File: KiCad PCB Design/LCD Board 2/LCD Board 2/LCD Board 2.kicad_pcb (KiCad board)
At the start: 2 copper layers, 27.9 x 27.9 mm, 8 parts, among them J1 Conn_01x03_Male, J2 Conn_01x03_Male, J3 Conn_01x02_Male, U1 ATtiny412-SS

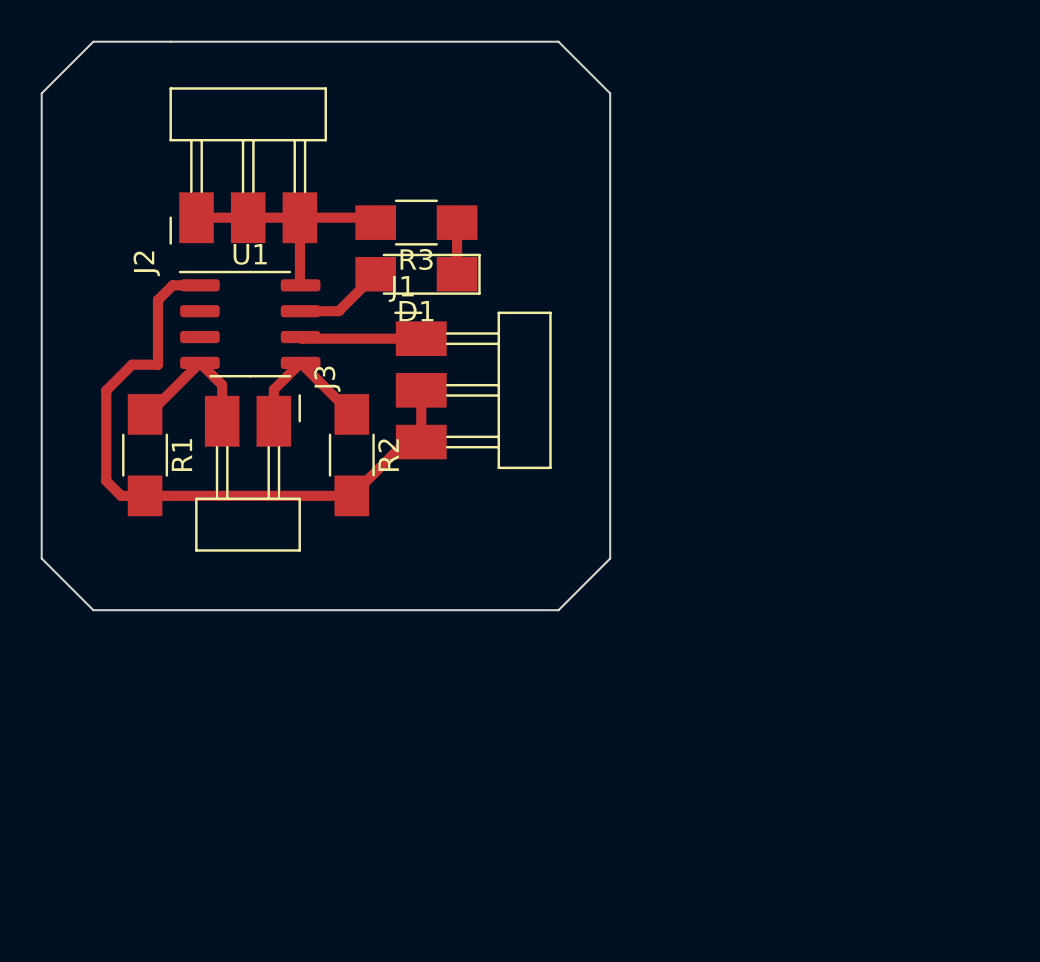
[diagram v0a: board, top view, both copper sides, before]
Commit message: v1.9 - KiCad LCD Board Updates
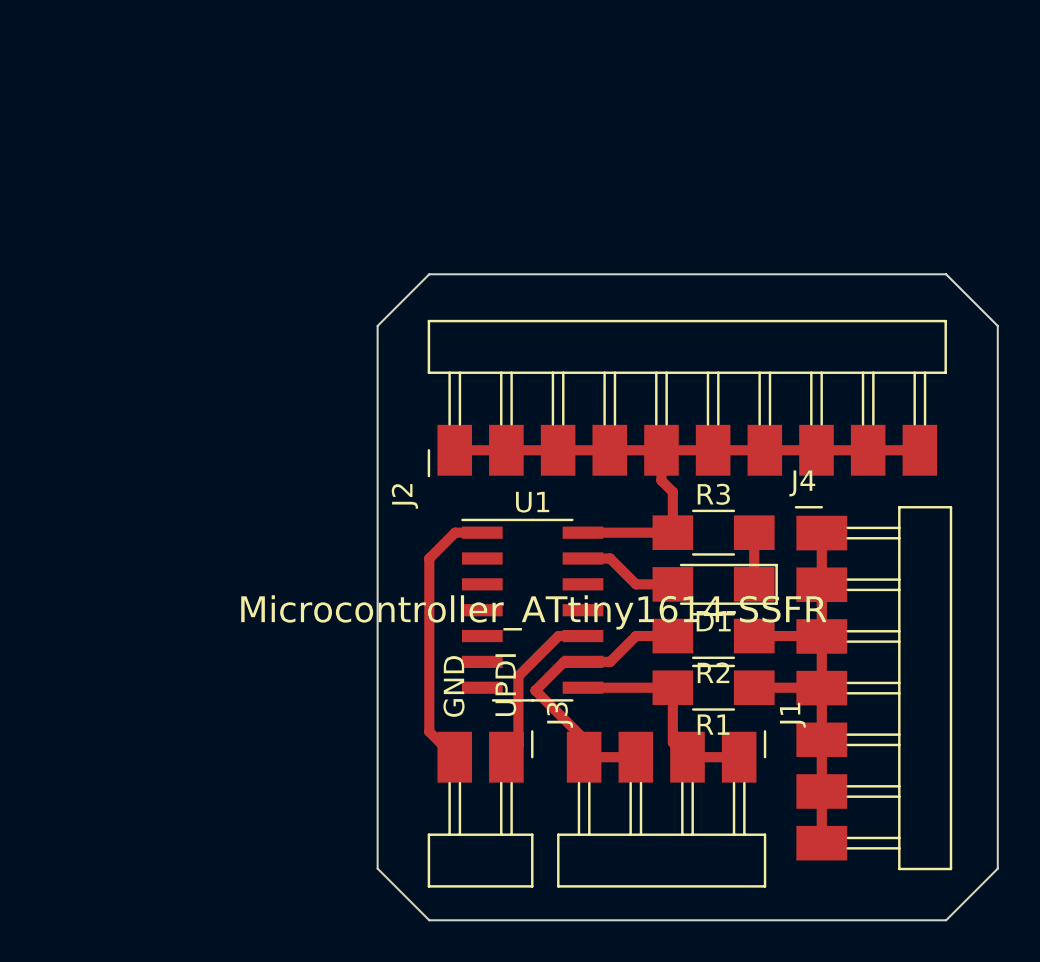
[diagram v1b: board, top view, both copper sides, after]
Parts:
- added J4: Conn_PinHeader_1x07_P2.54mm_Horizontal_SMD, fab:PinHeader_1x07_P2.54mm_Horizontal_SMD, F.Cu at (169.2, 118.1)
- J1: value Conn_01x03_Male -> Conn_PinHeader_1x04_P2.54mm_Horizontal_SMD; footprint fab:PinHeader_1x03_P2.54mm_Horizontal_SMD -> fab:PinHeader_1x04_P2.54mm_Horizontal_SMD
- J2: value Conn_01x03_Male -> Conn_PinHeader_1x10_P2.54mm_Horizontal_SMD; footprint fab:PinHeader_1x03_P2.54mm_Horizontal_SMD -> fab:PinHeader_1x10_P2.54mm_Horizontal_SMD
- J3: value Conn_01x02_Male -> Conn_PinHeader_1x02_P2.54mm_Horizontal_SMD; footprint fab:PinHeader_1x02_P2.54mm_Horizontal_SMD -> fab:PinHeader_UPDI_01x02_P2.54mm_Horizontal_SMD
- U1: value ATtiny412-SS -> Microcontroller_ATtiny1614-SSFR; footprint Package_SO:SOIC-8_3.9x4.9mm_P1.27mm -> fab:SOIC-14_3.9x8.7mm_P1.27mm
- moved R1 30.2 mm to (163.8, 125.7), turned to 180 degrees
- moved J1 25.8 mm to (165.1, 129.1), turned to -90 degrees
- moved D1 21.1 mm to (163.8, 120.7)
- moved R3 21.1 mm to (163.8, 118.1), turned to 0 degrees
- moved J3 20.1 mm to (153.7, 129.1)
- moved R2 19.9 mm to (163.8, 123.2), turned to 180 degrees
- moved U1 19.8 mm to (154.9, 121.9)
- moved J2 17.1 mm to (151.1, 114.1)
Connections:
- J1 pad 1: Net-(J1-Pad1) -> Net-(R1-Pad2)
- J1 pad 2: Net-(J1-Pad2) -> Net-(R1-Pad2)
- J1 pad 3: Net-(J1-Pad2) -> Net-(J1-Pad3)
- J2 pad 1: Net-(J2-Pad1) -> Net-(R3-Pad1)
- J2 pad 2: Net-(J2-Pad1) -> Net-(R3-Pad1)
- J2 pad 3: Net-(J2-Pad1) -> Net-(R3-Pad1)
- R1 pad 1: Net-(J3-Pad2) -> Net-(R1-Pad1)
- R1 pad 2: Net-(J1-Pad2) -> Net-(R1-Pad2)
- R2 pad 1: Net-(J3-Pad1) -> Net-(R1-Pad1)
- R2 pad 2: Net-(J1-Pad2) -> Net-(J1-Pad3)
- R3 pad 1: Net-(D1-Pad1) -> Net-(R3-Pad1)
- R3 pad 2: Net-(J2-Pad1) -> Net-(D1-Pad1)
- U1 pad 1: Net-(J1-Pad2) -> Net-(J3-Pad2)
- U1 pad 4: Net-(J3-Pad2) -> unconnected-(U1-Pad4)
- U1 pad 5: Net-(J3-Pad1) -> unconnected-(U1-Pad5)
- U1 pad 6: Net-(J1-Pad1) -> unconnected-(U1-Pad6)
- U1 pad 7: Net-(D1-Pad2) -> unconnected-(U1-Pad7)
- U1 pad 8: Net-(J2-Pad1) -> Net-(R1-Pad2)
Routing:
- net Net-(J1-Pad2): track 32.5 -> 0.00 mm
- net Net-(R3-Pad1): track 0.00 -> 31.6 mm
- net Net-(R1-Pad1): track 0.00 -> 21.9 mm
- net Net-(J1-Pad3): track 0.00 -> 14.7 mm
- net Net-(J2-Pad1): track 12.2 -> 0.00 mm
- net Net-(R1-Pad2): track 0.00 -> 10.7 mm
- net Net-(J3-Pad2): track 7.07 -> 13.4 mm
- net Net-(J1-Pad1): track 5.96 -> 0.00 mm
- net Net-(J3-Pad1): track 6.99 -> 8.22 mm
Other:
- board size 27.9 x 27.9 mm -> 30.5 x 31.8 mm
